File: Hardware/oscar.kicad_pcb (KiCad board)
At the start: 4 copper layers, 71 x 110 mm, 51 parts, among them J1 SWD_Header, J2 ChannelA_In, J3 ChannelB_In, J4 ChannelC_In, J5 ChA_Buff_Out, J6 ChB_Buff_Out, J7 ChC_Buff_Out, J8 MIDI_In, J9 Eurorack_10_pin_power, SW1 Left_Encoder, SW2 Right_Encoder, SW3 SW_Push, U1 STM32F446RETx, U2 ILI9341_SPI_Daughterboard, U3 MCP6004, U4 TL074, U5 LM1117-3.3, Y1 Crystal

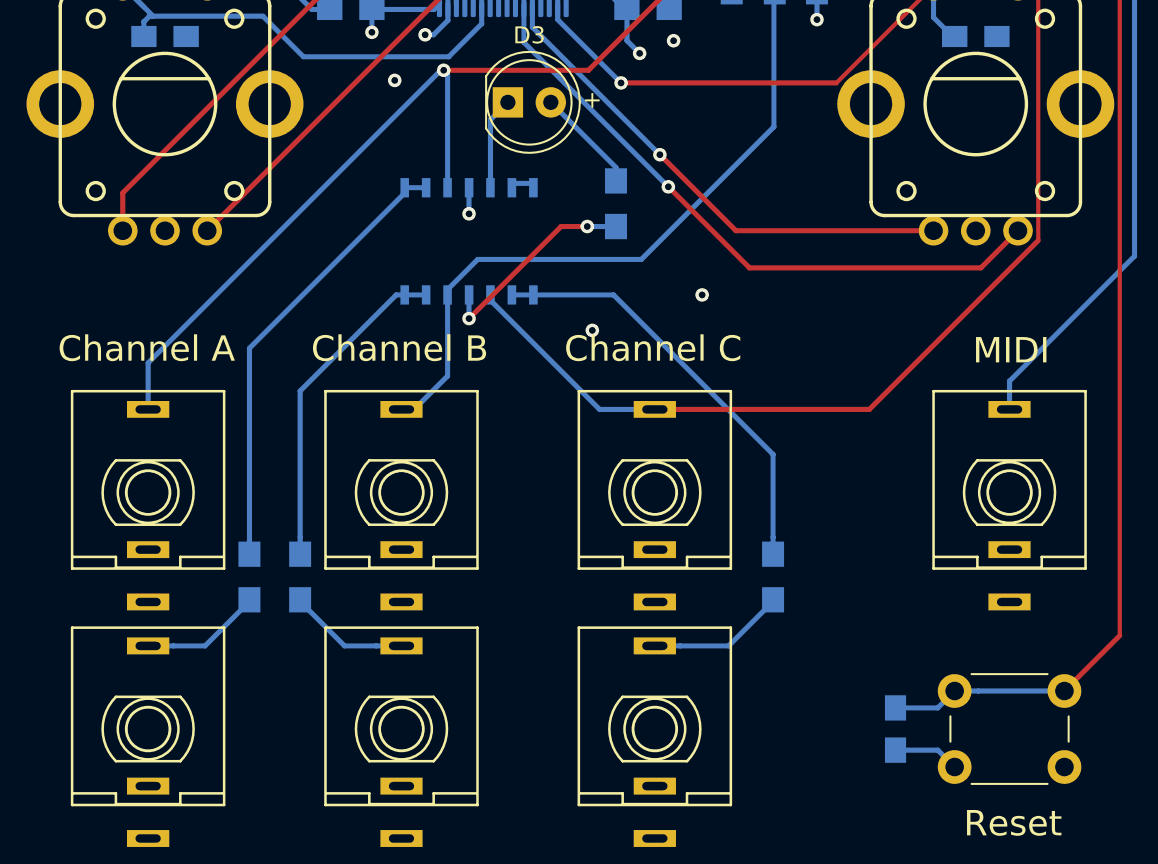
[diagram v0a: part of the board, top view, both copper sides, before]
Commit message: Added readme and graphics
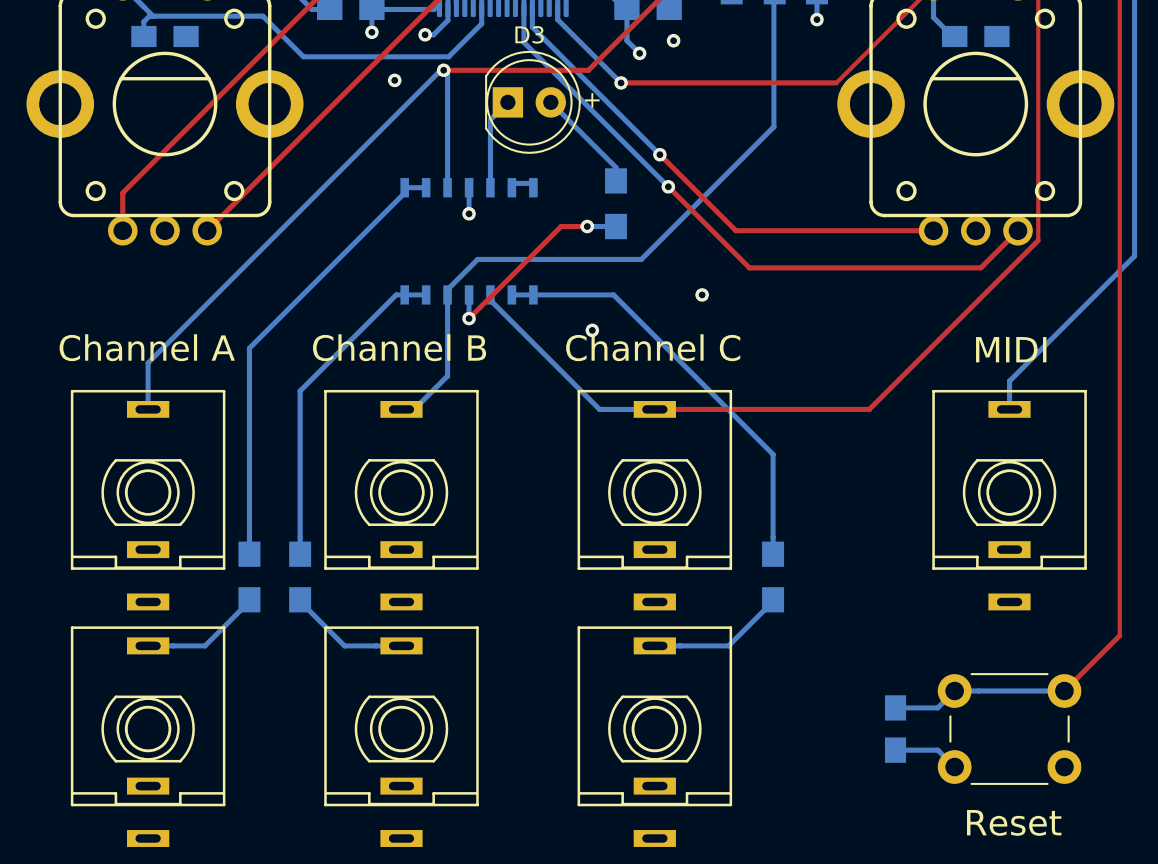
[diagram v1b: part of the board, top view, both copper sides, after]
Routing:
- added copper zone on In2.Cu, net +3V3
- added copper zone on In1.Cu, net GND
- added copper zone on In2.Cu, net VCC
- added copper zone on In2.Cu, net VEE
- removed copper zone on PWR, net +3V3
- removed copper zone on GND, net GND
- removed copper zone on PWR, net VCC
- removed copper zone on PWR, net VEE
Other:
- net class Default removed
